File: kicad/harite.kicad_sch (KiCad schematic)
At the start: 48 parts, among them J1 59453-121110ECHLF, J2 59453-051110ECHLF, J3 59453-051110ECHLF, J4 59453-081110EDHLF, J5 59453-081110EDHLF, U1 RP2040_Zero

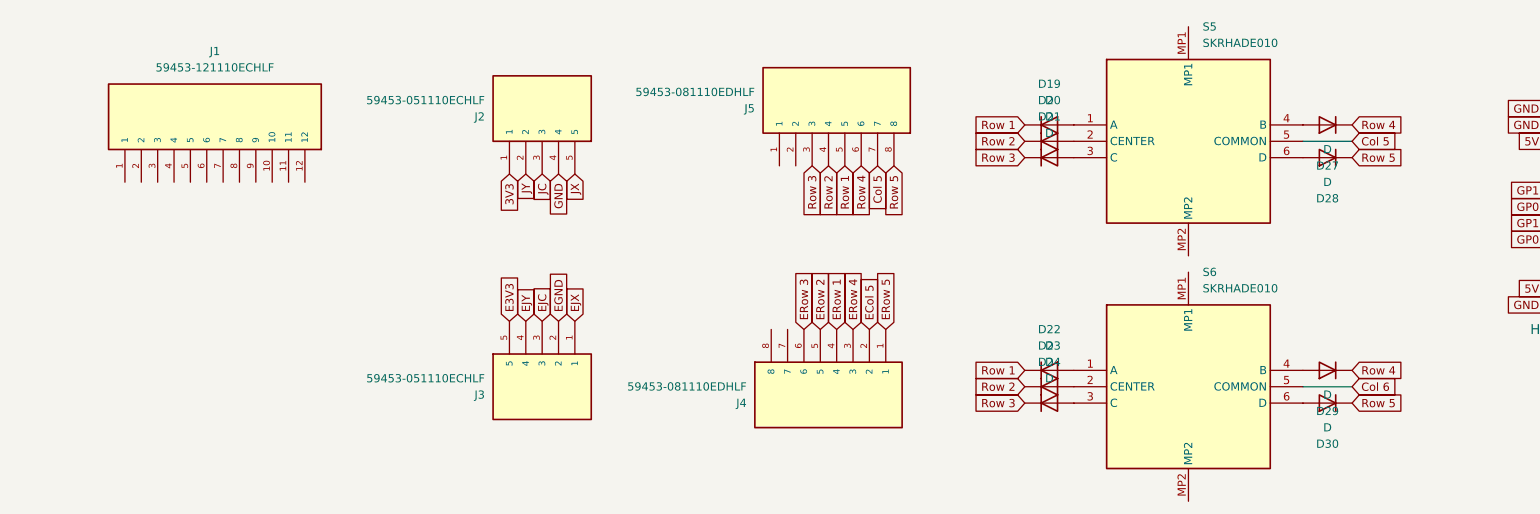
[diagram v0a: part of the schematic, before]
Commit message: Update nets
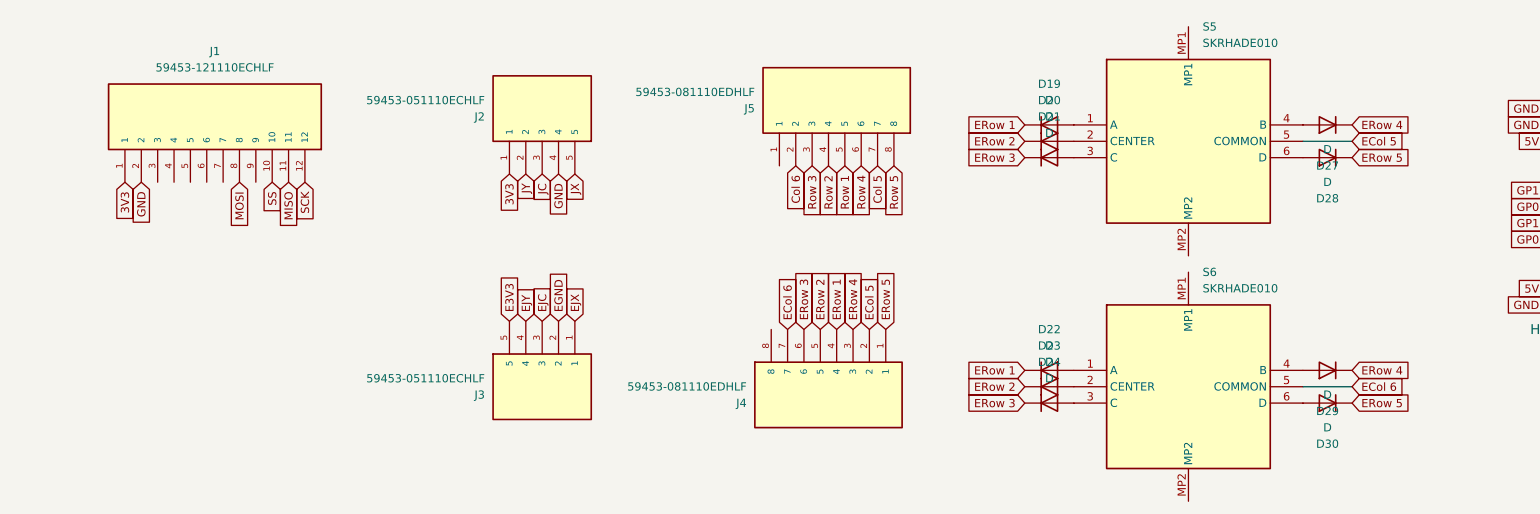
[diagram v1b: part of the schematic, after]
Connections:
- net 3V3: now also J1.1
- net Col 5: no longer S5.5 (COMMON)
- net Col 6: now also J5.2; no longer S6.5 (COMMON)
- net ECol 5: now also S5.5 (COMMON)
- net ERow 1: now also D19.1 (K), D22.1 (K)
- net ERow 2: now also D20.1 (K), D23.1 (K)
- net ERow 3: now also D21.1 (K), D24.1 (K)
- net ERow 4: now also D27.1 (K), D29.1 (K)
- net ERow 5: now also D28.1 (K), D30.1 (K)
- net GND: now also J1.2
- net MISO: now also J1.11
- net MOSI: now also J1.8
- net Row 1: no longer D19.1 (K), D22.1 (K)
- net Row 2: no longer D20.1 (K), D23.1 (K)
- net Row 3: no longer D21.1 (K), D24.1 (K)
- net Row 4: no longer D27.1 (K), D29.1 (K)
- net Row 5: no longer D28.1 (K), D30.1 (K)
- net SCK: now also J1.12
- net SS: now also J1.10
- net ECol 6: now reaches J4.7
- net ECol 6: now also S6.5 (COMMON)
